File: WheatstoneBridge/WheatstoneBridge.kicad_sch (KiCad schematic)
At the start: 6 parts

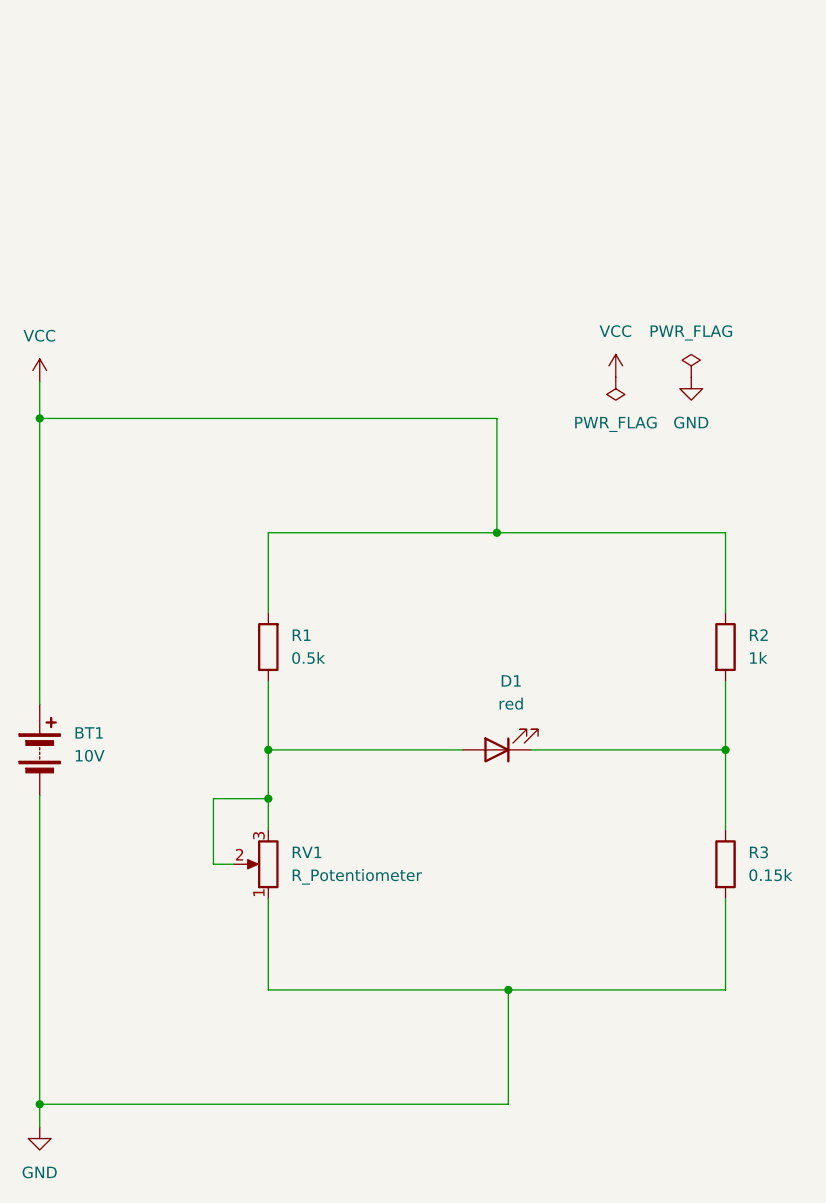
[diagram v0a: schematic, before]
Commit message: Update wheatstonebridges
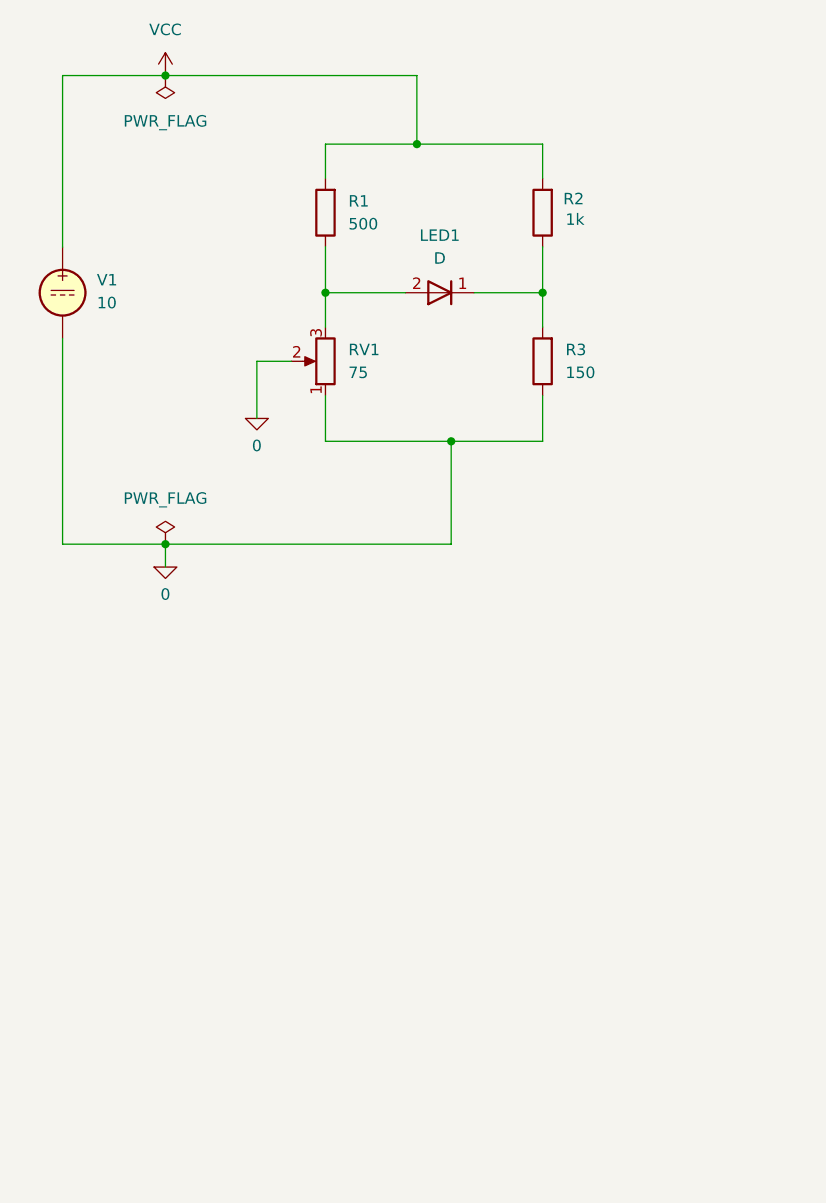
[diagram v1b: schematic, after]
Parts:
- removed BT1: 10V, Battery:BatteryHolder_Keystone_1060_1x2032, symbol Device:Battery
- removed D1: red, LED_THT:LED_D5.0mm, symbol Device:LED
- added LED1: D, symbol Simulation_SPICE:D
- added V1: 10, symbol Simulation_SPICE:VDC
- R1: value 0.5k -> 500
- R3: value 0.15k -> 150
- RV1: value R_Potentiometer -> 75
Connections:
- net VCC: now also R2.2, V1.1; no longer R2.1
- net at R1.1, RV1.3: now also LED1.2 (A); no longer RV1.2
- net 0: now reaches R3.1
- net 0: now also RV1.1, RV1.2, V1.2; no longer R2.2
- net GND: no longer names the net of R3.2
- net GND: now also R2.1, LED1.1 (K); no longer RV1.1
